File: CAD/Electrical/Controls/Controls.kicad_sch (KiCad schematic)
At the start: 59 parts, among them J1 Aileron Servo, J10 Battery and/or BMS, J11 Restart/Boot Button, J12 GPS, J13 Cadence Sensor, J14 Gyroscope, J15 LCD, J16 pitot tube assembly, J17 SD card selecting jumper, J18 SD card selecting jumper, J19 Aileron Servo, J2 SD card, J20 Elevator Servo, J3 External Connector, J4 Rudder Servo, J5 Elevator Servo, J6 BME280, J7 Pitch Control, J8 Roll Control, J9 SD card selecting jumper, U1 ESP32-C3-DevKitM-1, U2 5V regulator, U3 6V regulator, U4 6V regulator, U5 6V regulator, U6 6V regulator, U7 6V regulator, U8 3V3 regulator, U9 ESP32-WROOM-32E

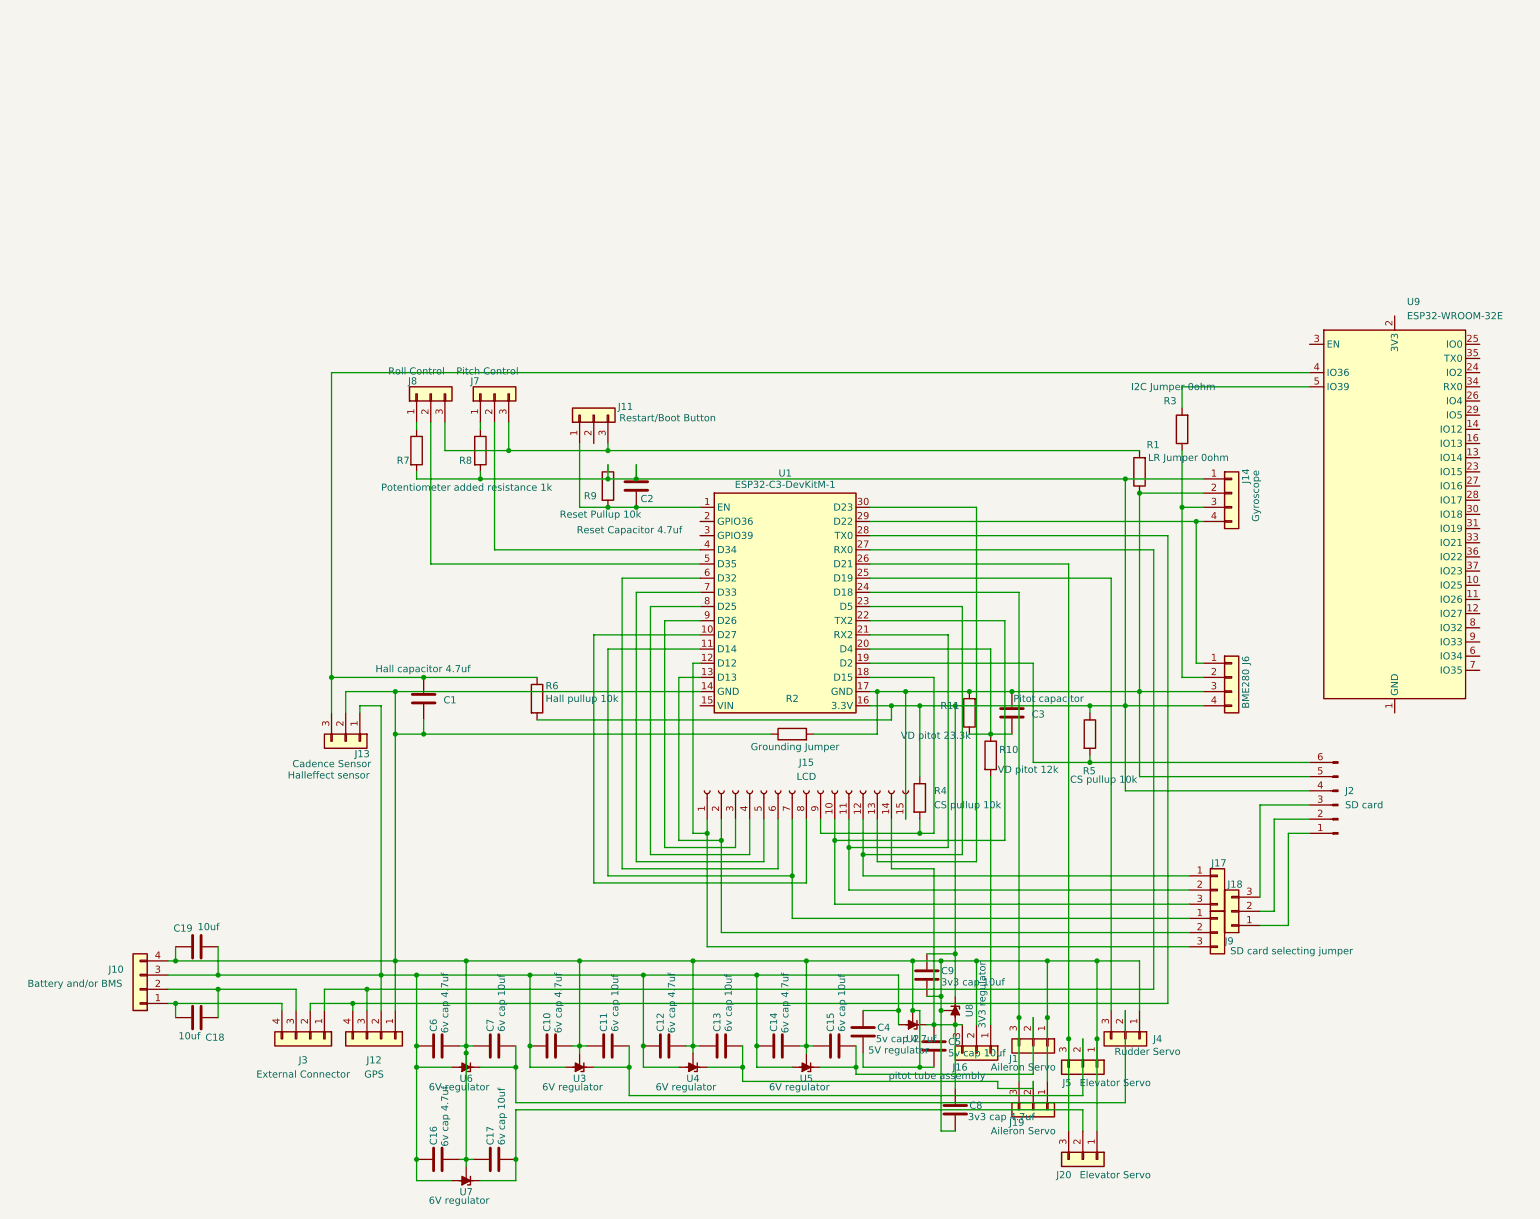
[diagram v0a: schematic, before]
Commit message: Schematic and almost BOM
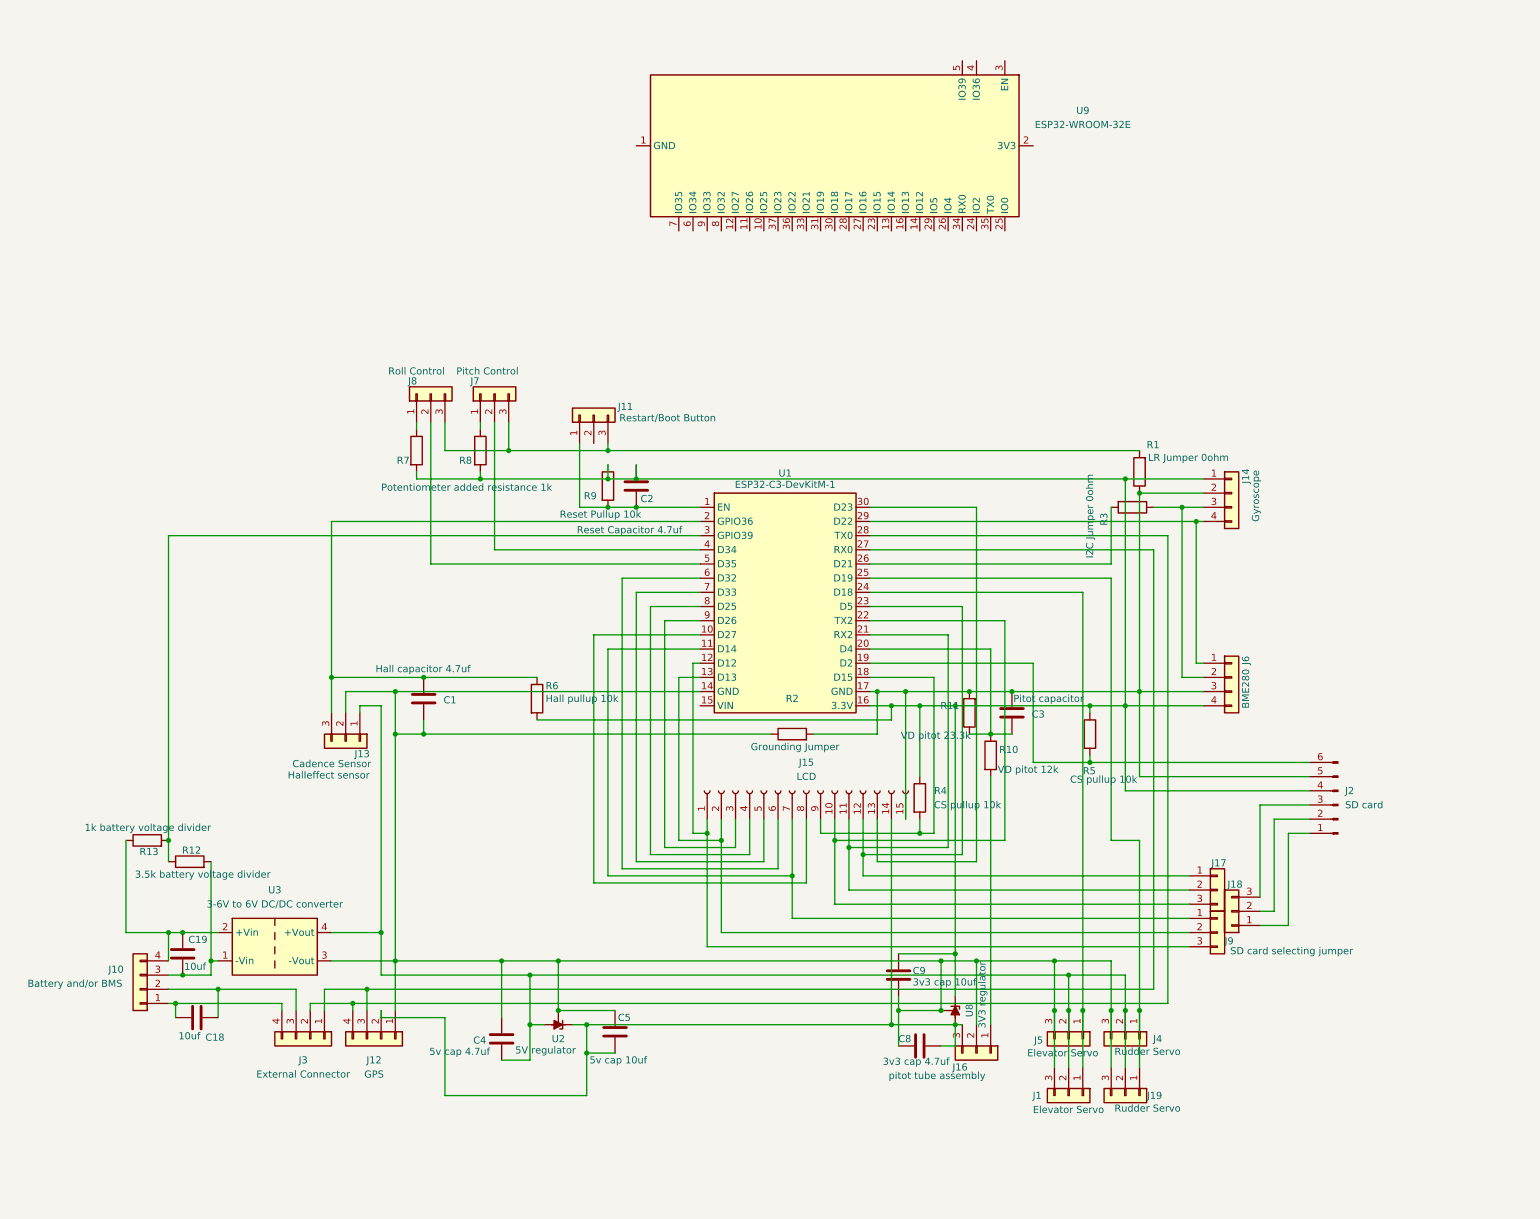
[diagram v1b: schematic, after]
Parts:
- removed C10, C12, C14, C16, C6: 6v cap 4.7uf, Capacitor_SMD:C_0402_1005Metric_Pad0.74x0.62mm_HandSolder, symbol Device:C
- removed C11, C13, C15, C17, C7: 6v cap 10uf, Capacitor_SMD:C_0402_1005Metric_Pad0.74x0.62mm_HandSolder, symbol Device:C
- removed J20: Elevator Servo, Connector_Molex:Molex_KK-254_AE-6410-03A_1x03_P2.54mm_Vertical, symbol Connector_Generic:Conn_01x03
- removed U3, U4, U5, U6, U7: 6V regulator, Package_TO_SOT_SMD:TO-252-2, symbol Reference_Voltage:TL431KTP
- added R12: 3.5k battery voltage divider, symbol Device:R
- added R13: 1k battery voltage divider, symbol Device:R
- added U3: 3-6V to 6V DC/DC converter, Converter_DCDC:Converter_DCDC_TRACO_TMU3-05xx_12xx_THT, symbol Converter_DCDC:TMU3-1212
- J1: value Aileron Servo -> Elevator Servo
- J19: value Aileron Servo -> Rudder Servo
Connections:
- net at C1.2, C9.2, J12.1 (Pin_1)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: now also C4.1, C5.1, C8.1, J1.3 (Pin_3), J19.3 (Pin_3), J4.3 (Pin_3), J5.3 (Pin_3), U3.3 (-Vout); no longer C19.1, C4.2, C5.2, C8.2, J1.1 (Pin_1), J10.4 (Pin_4), J19.1 (Pin_1), J4.1 (Pin_1), J5.1 (Pin_1)
- net at J19.2 (Pin_2): now also C4.2, J1.2 (Pin_2), J13.1 (Pin_1), J4.2 (Pin_2), J5.2 (Pin_2), U2.2 (A), U3.4 (+Vout)
- net at J15.14 (Pin_14), J16.3 (Pin_3), U2.3 (K)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: now also C5.2, C8.2, J12.2 (Pin_2); no longer C5.1, C8.1
- net at C1.1, J13.3 (Pin_3), R6.1: now also U1.2 (GPIO36); no longer U9.4 (IO36)
- net at R3.2: now also U1.26 (D21); no longer U9.5 (IO39)
- net at U1.25 (D19): now also J19.1 (Pin_1), J4.1 (Pin_1); no longer J4.3 (Pin_3)
- net at U1.3 (GPIO39): now also R12.1, R13.2
- new net: J1.1 (Pin_1), J5.1 (Pin_1), U1.24 (D18)
- new net: C19.1, J10.4 (Pin_4), R13.1, U3.2 (+Vin)
- new net: C19.2, J10.3 (Pin_3), R12.2, U3.1 (-Vin)
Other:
- moved on the sheet: C19, C4, C5, C8, C9, J5, R3, U2, U9

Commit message: schematics and weight update
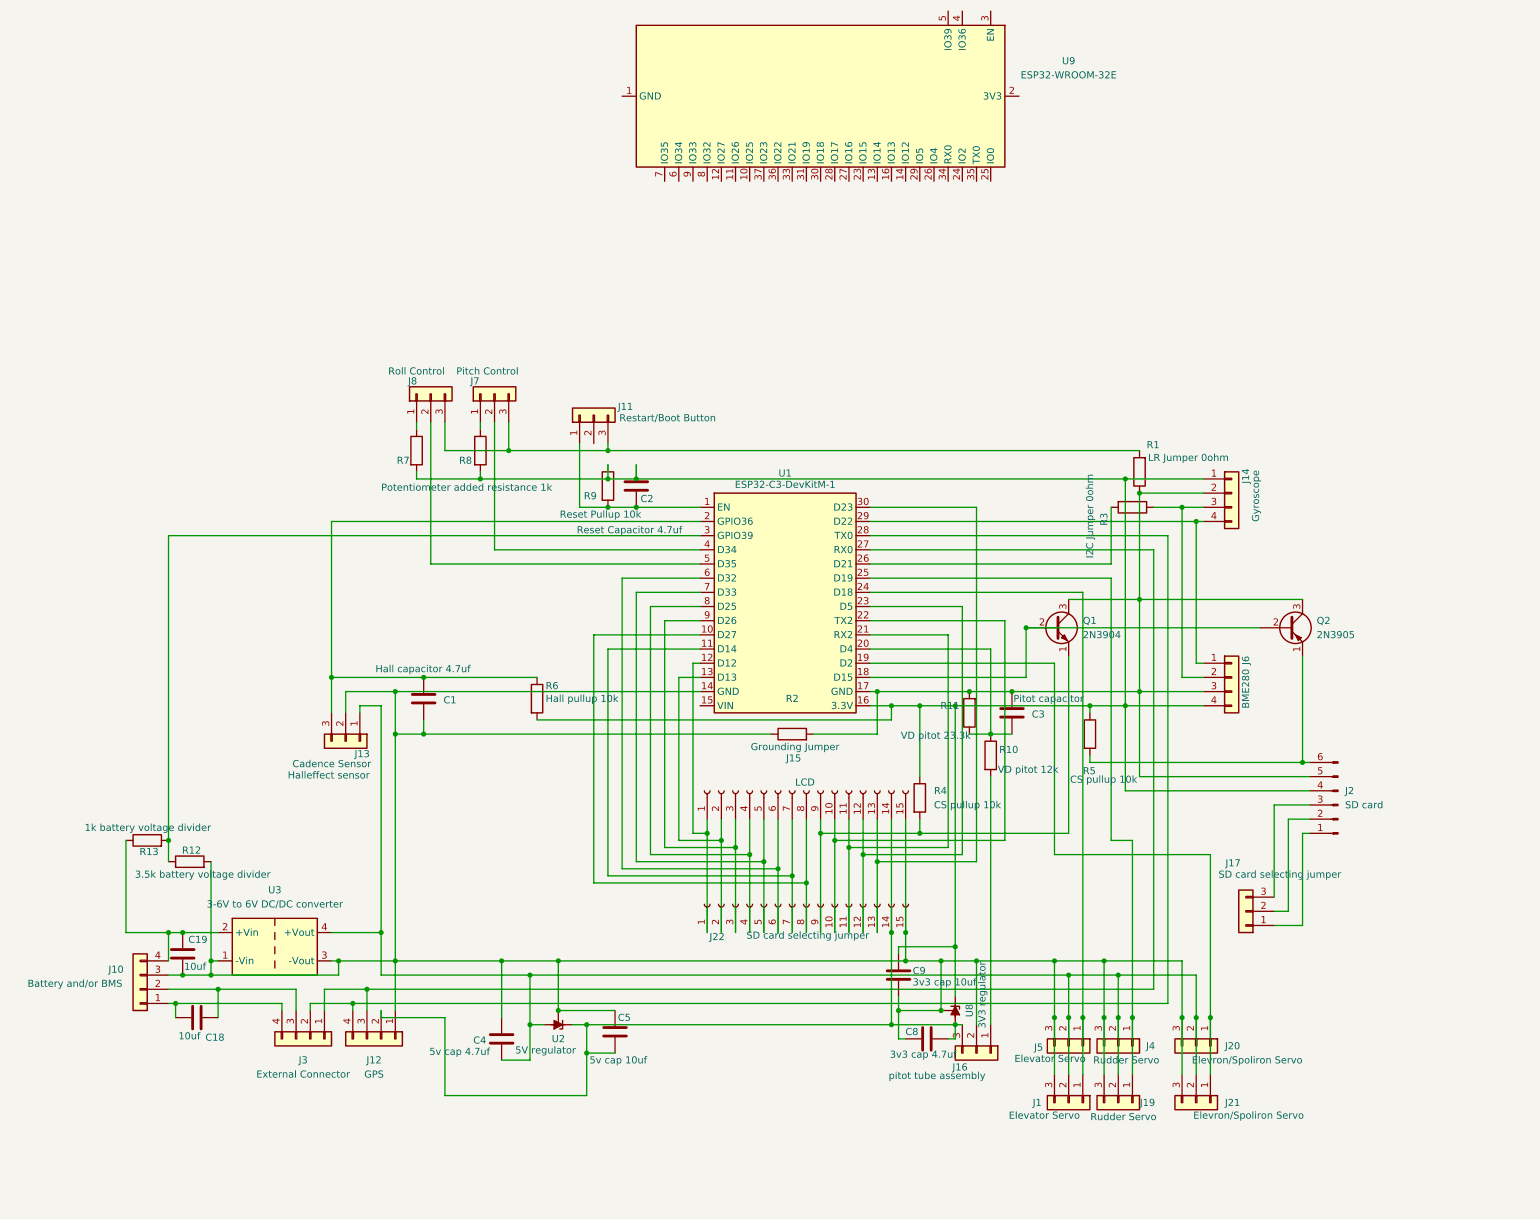
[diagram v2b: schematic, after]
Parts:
- removed J18, J9: SD card selecting jumper, symbol Connector_Generic:Conn_01x03
- added J20, J21: Elevron/Spoliron Servo, Connector_Molex:Molex_KK-254_AE-6410-03A_1x03_P2.54mm_Vertical, symbol Connector_Generic:Conn_01x03
- added J22: SD card selecting jumper, Connector_Hirose:Hirose_DF13-15P-1.25DSA_1x15_P1.25mm_Vertical, symbol Connector:Conn_01x15_Socket
- added Q1: 2N3904, Package_TO_SOT_THT:TO-92_Inline, symbol Transistor_BJT:2N3904
- added Q2: 2N3905, Package_TO_SOT_THT:TO-92_Inline, symbol Transistor_BJT:2N3905
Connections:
- net at C3.1, J14.2 (Pin_2), J2.5 (Pin_5)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: now also Q1.3 (C), Q2.3 (C); no longer J15.15 (Pin_15)
- net at C1.2, C4.1, C5.1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: now also C19.2, J10.3 (Pin_3), J15.15 (Pin_15), R12.2, U3.1 (-Vin), J20.3 (Pin_3), J21.3 (Pin_3), J22.15 (Pin_15)
- net at C5.2, C8.2, J12.2 (Pin_2)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: now also J22.14 (Pin_14)
- net at J15.1 (Pin_1), U1.12 (D12): now also J22.1 (Pin_1)
- net at J15.10 (Pin_10), U1.22 (TX2): now also J22.10 (Pin_10)
- net at J15.11 (Pin_11), U1.21 (RX2): now also J22.11 (Pin_11)
- net at J15.12 (Pin_12), U1.23 (D5): now also J22.12 (Pin_12)
- net at J15.13 (Pin_13), U1.30 (D23): now also J22.13 (Pin_13)
- net at J15.2 (Pin_2), U1.13 (D13): now also J22.2 (Pin_2)
- net at J15.3 (Pin_3), U1.9 (D26): now also J22.3 (Pin_3)
- net at J15.4 (Pin_4), U1.8 (D25): now also J22.4 (Pin_4)
- net at J15.5 (Pin_5), U1.7 (D33): now also J22.5 (Pin_5)
- net at J15.6 (Pin_6), U1.6 (D32): now also J22.6 (Pin_6)
- net at J15.7 (Pin_7), U1.11 (D14): now also J22.7 (Pin_7)
- net at J15.8 (Pin_8), U1.10 (D27): now also J22.8 (Pin_8)
- net at J15.9 (Pin_9), R4.2: now also J22.9 (Pin_9), Q1.1 (E); no longer U1.18 (D15)
- net at C4.2, J1.2 (Pin_2), J13.1 (Pin_1)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: now also J20.2 (Pin_2), J21.2 (Pin_2)
- net at J2.6 (Pin_6), R5.2: now also Q2.1 (E); no longer U1.19 (D2)
- new net: J20.1 (Pin_1), J21.1 (Pin_1), U1.19 (D2)
- new net: Q1.2 (B), Q2.2 (B), U1.18 (D15)
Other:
- moved on the sheet: C8, J1, J17, J19, J4, J5, U9
